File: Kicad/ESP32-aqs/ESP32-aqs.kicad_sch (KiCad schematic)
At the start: 28 parts, among them J1 UART Connector, J2 JST connector SEN55, J3 ufl connector, SW1 RESET, SW2 BOOT, U1 LD1117S33TR_SOT223, U2 ESP32-WROOM-32, U3 SGP41-D-R4, U4 SX1276S8S+T-X1

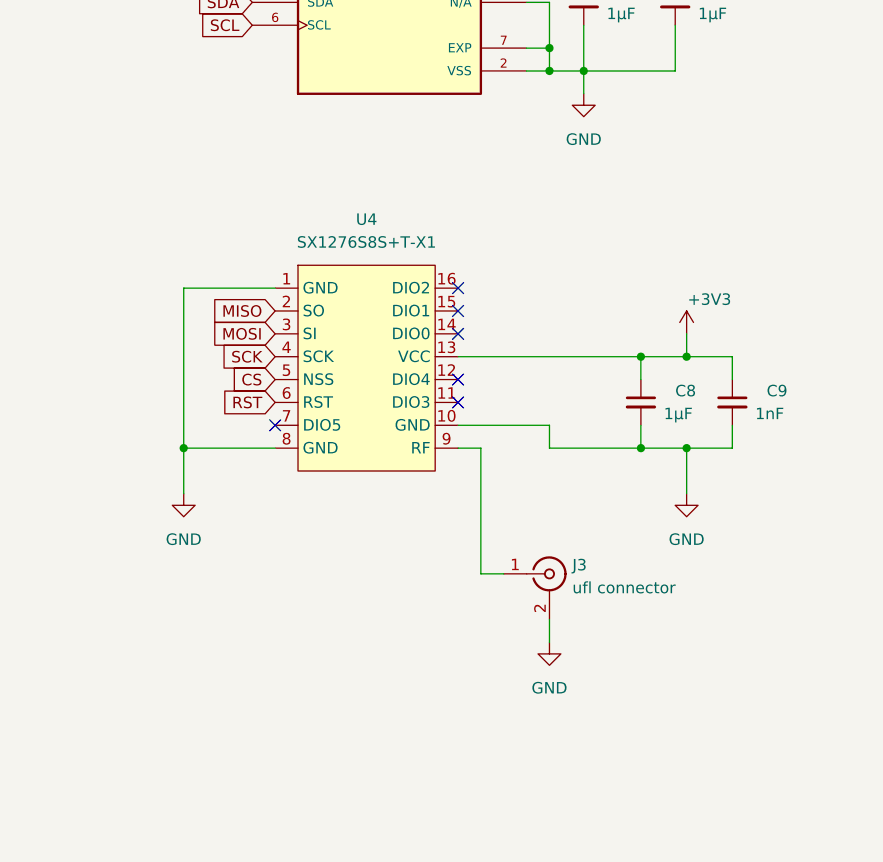
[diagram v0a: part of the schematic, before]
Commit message: PCB design
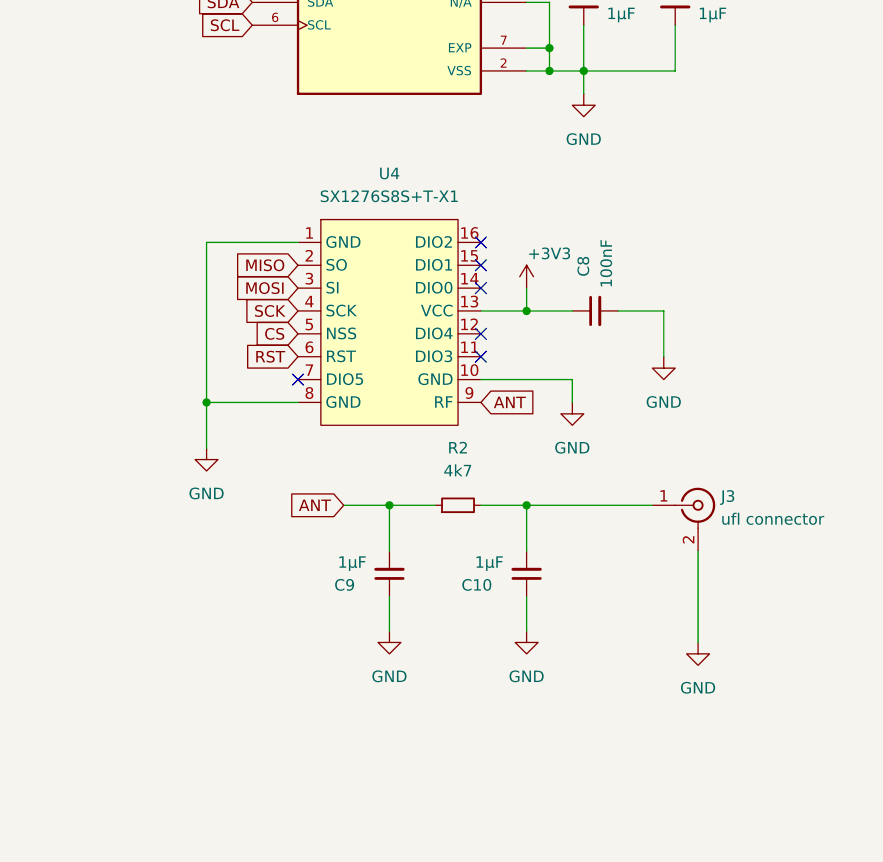
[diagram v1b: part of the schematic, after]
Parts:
- added C10: 1µF, Capacitor_SMD:C_0805_2012Metric_Pad1.18x1.45mm_HandSolder, symbol Device:C_Small
- added R2: 4k7, Resistor_SMD:R_0805_2012Metric_Pad1.20x1.40mm_HandSolder, symbol Device:R_Small
- C8: value 1µF -> 100nF
- C9: value 1nF -> 1µF
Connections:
- net +3V3: no longer C9.1
- net GND: now also C9.1, C10.1; no longer C9.2
- net at J3.1 (In): now also C10.2, R2.2; no longer U4.9 (RF)
- new net ANT: C9.2, R2.1, U4.9 (RF)
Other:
- moved on the sheet: C8, J3, U4

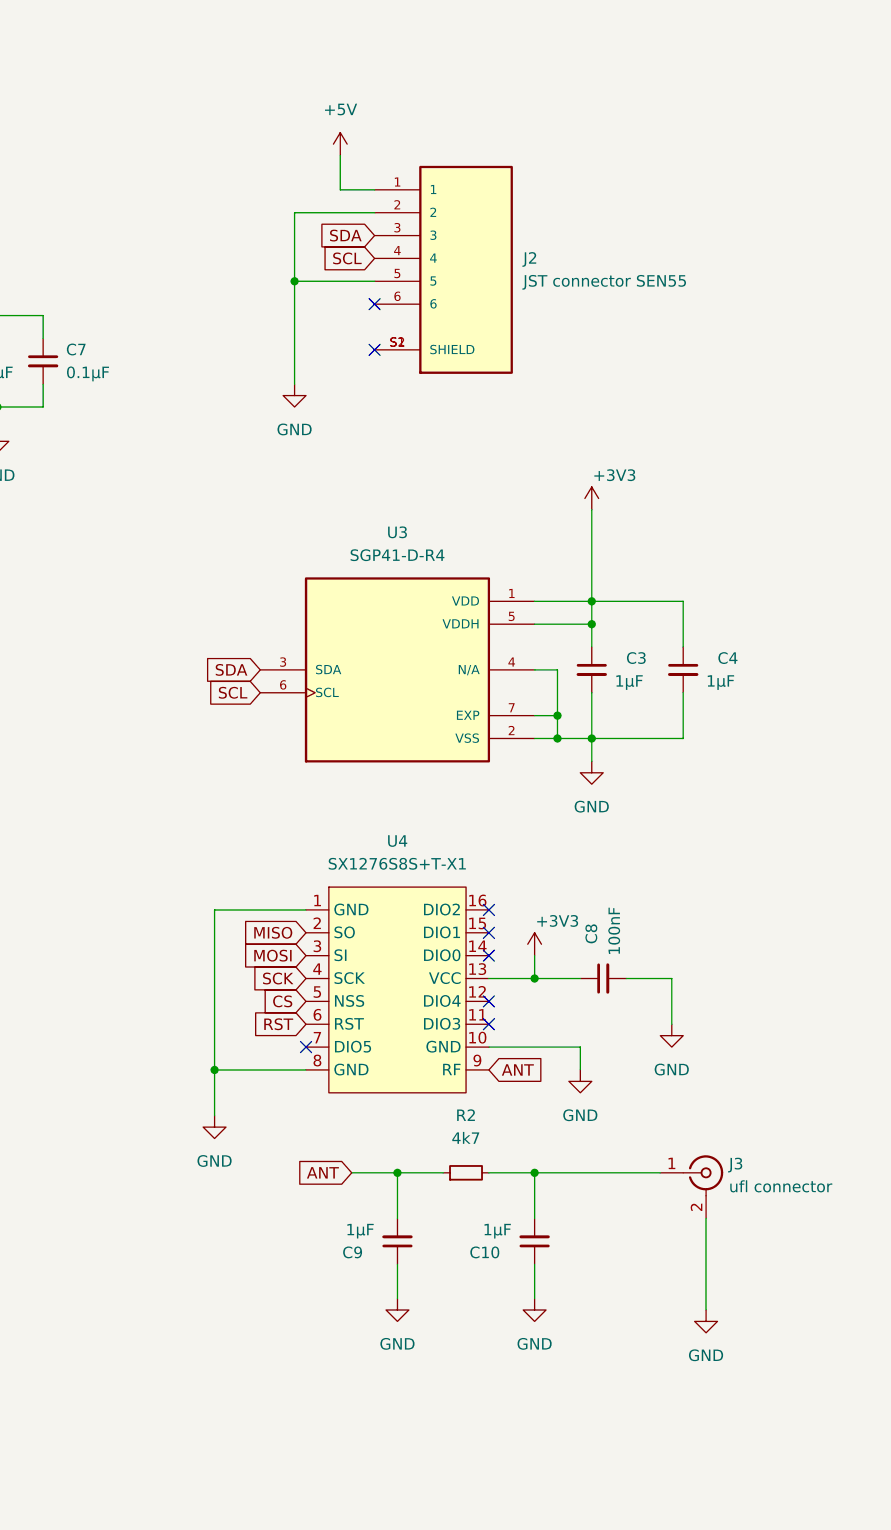
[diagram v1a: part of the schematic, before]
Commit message: PCB + BoM
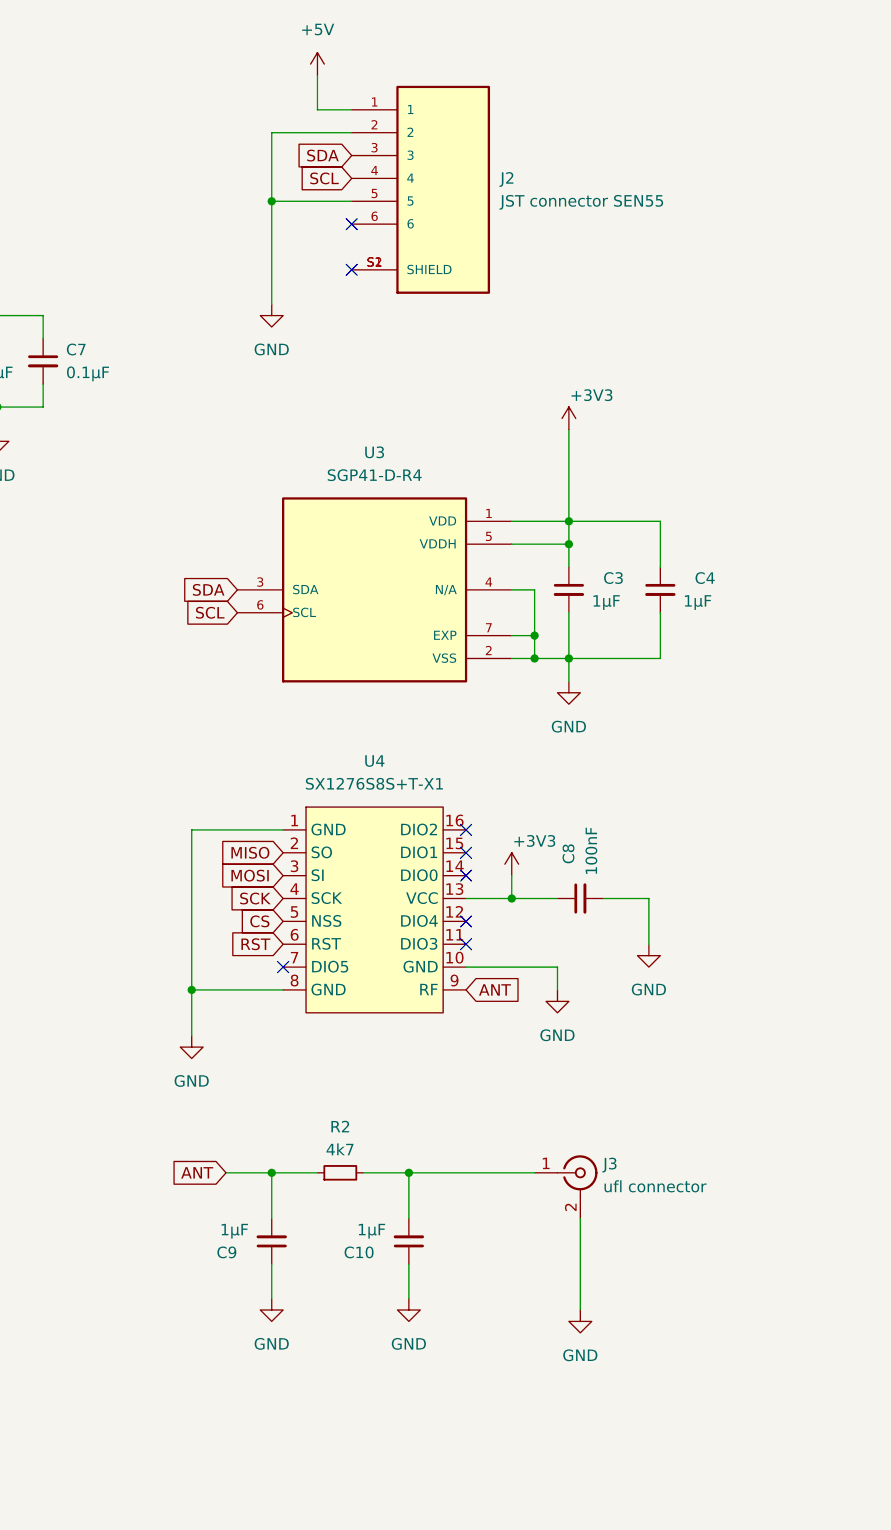
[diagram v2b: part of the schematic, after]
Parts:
- U2: LCSC (none) -> C718834
- U4: LCSC (none) -> C2844472
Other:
- moved on the sheet: C10, C3, C4, C8, C9, J2, J3, R2, U3, U4
